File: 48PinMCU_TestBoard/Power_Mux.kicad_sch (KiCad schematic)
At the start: 8 parts, among them U4 TPS2117DRLR

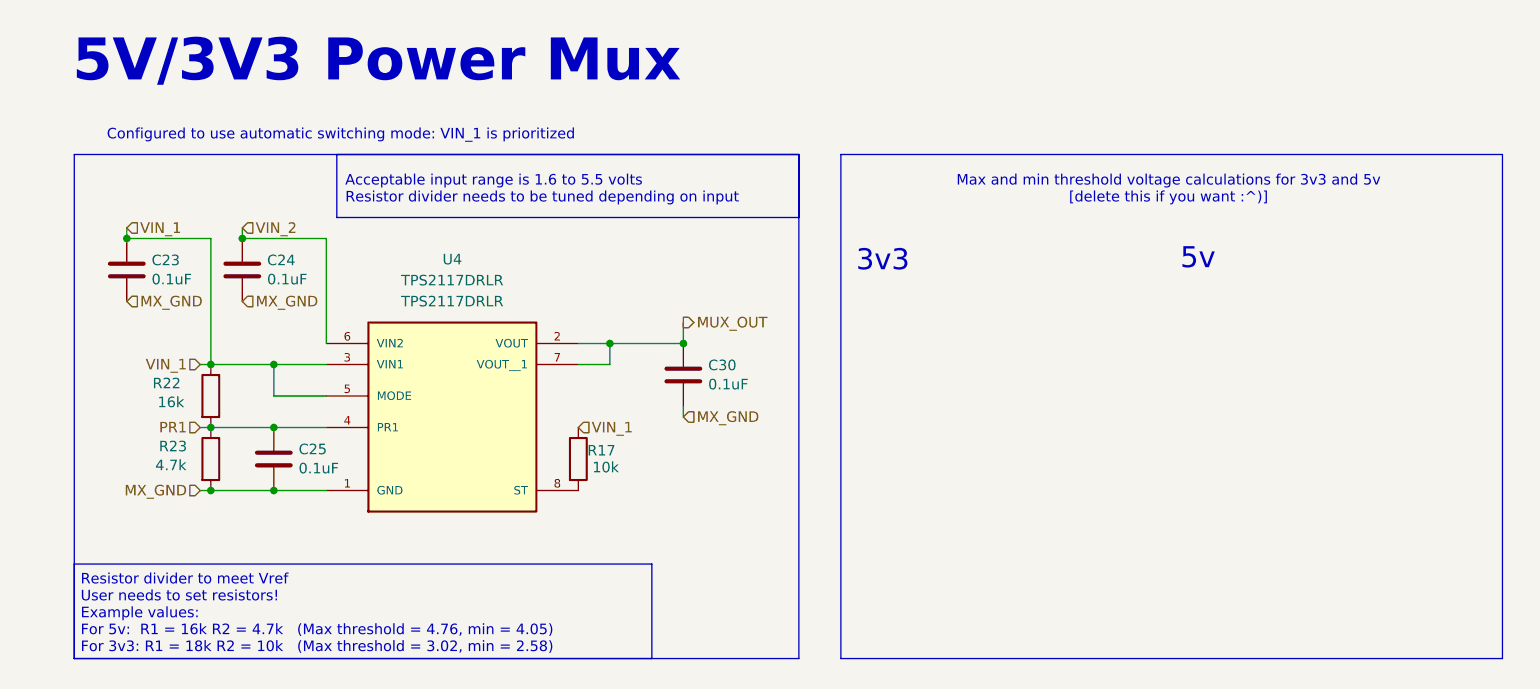
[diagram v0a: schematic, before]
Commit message: All fixes fixed
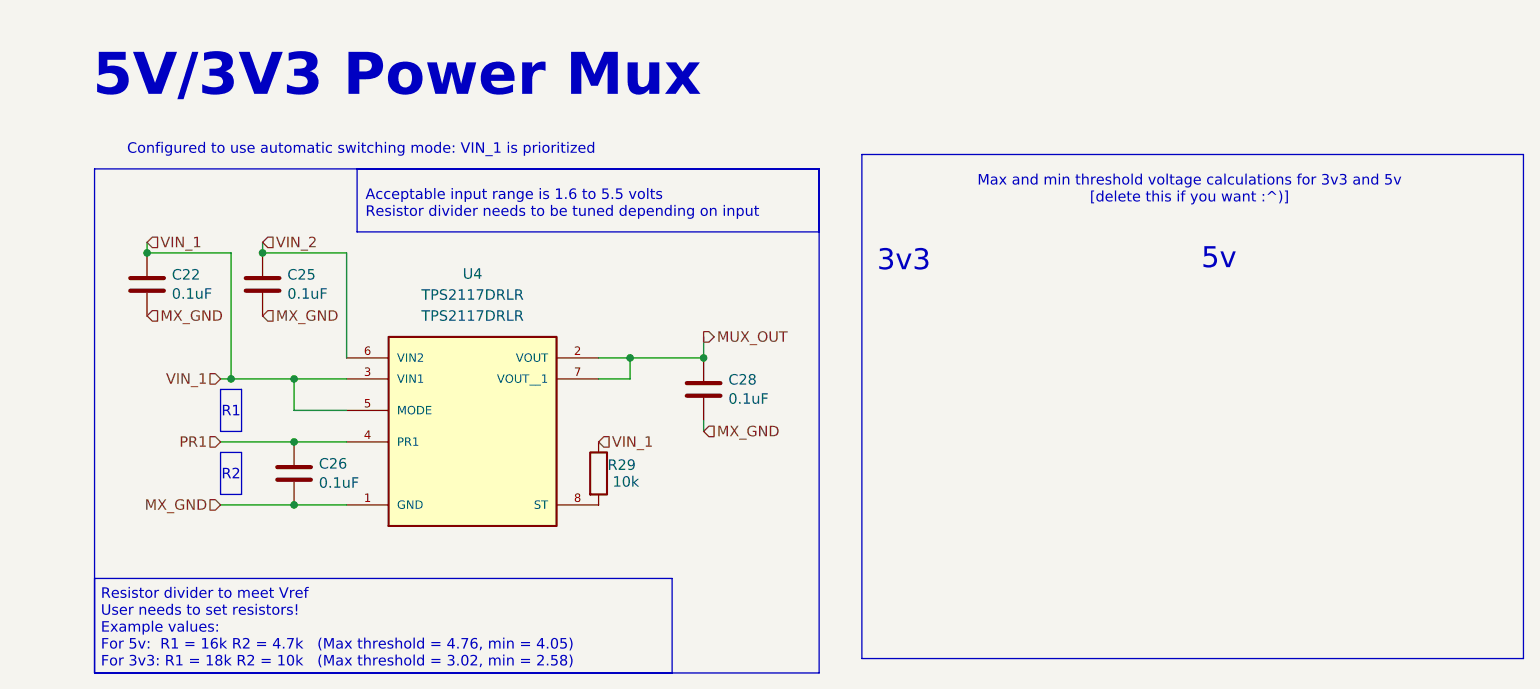
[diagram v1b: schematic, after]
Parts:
- removed C23, C25, C30: 0.1uF, Capacitor_SMD:C_0603_1608Metric_Pad1.08x0.95mm_HandSolder, symbol Device:C
- removed R17: 10k, Resistor_SMD:R_0603_1608Metric_Pad0.98x0.95mm_HandSolder, symbol Device:R
- removed R22: 16k, Resistor_SMD:R_0603_1608Metric_Pad0.98x0.95mm_HandSolder, symbol Device:R
- removed R23: 4.7k, Resistor_SMD:R_0603_1608Metric_Pad0.98x0.95mm_HandSolder, symbol Device:R
- added C22, C26, C28: 0.1uF, Capacitor_SMD:C_0603_1608Metric_Pad1.08x0.95mm_HandSolder, symbol Device:C
- added R29: 10k, Resistor_SMD:R_0603_1608Metric_Pad0.98x0.95mm_HandSolder, symbol Device:R
- U4: LCSC P/N C22399676 -> (none)
- renumbered C24 to C25
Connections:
- net MUX_OUT: now also C28.1
- net MX_GND: now also C22.2, C26.2, C28.2
- net PR1: now also C26.1
- net VIN_1: now also C22.1, R29.1
- net at U4.8 (ST): now also R29.2
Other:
- note added: "R1"
- note added: "R2"
- moved on the sheet: C25

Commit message: preliminary layout blocks
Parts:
- R29: LCSC P/N (none) -> C25804
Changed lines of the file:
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@@
+			)
+		)
+		(property "LCSC P/N" "C25804"
+			(at 81.1893 72.8625 0)
+			(effects
+				(font
+					(size 1.27 1.27)
+				)
+				(hide yes)
 			)
 		)
